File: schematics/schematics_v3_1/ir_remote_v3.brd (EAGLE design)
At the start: 77.5 x 49.5 mm, 26 parts, among them IC1 AP1117E50G, Q1 10MHz, T11 TASTER3301, T12 TASTER3301, T13 TASTER3301, T14 TASTER3301, T15 TASTER3301

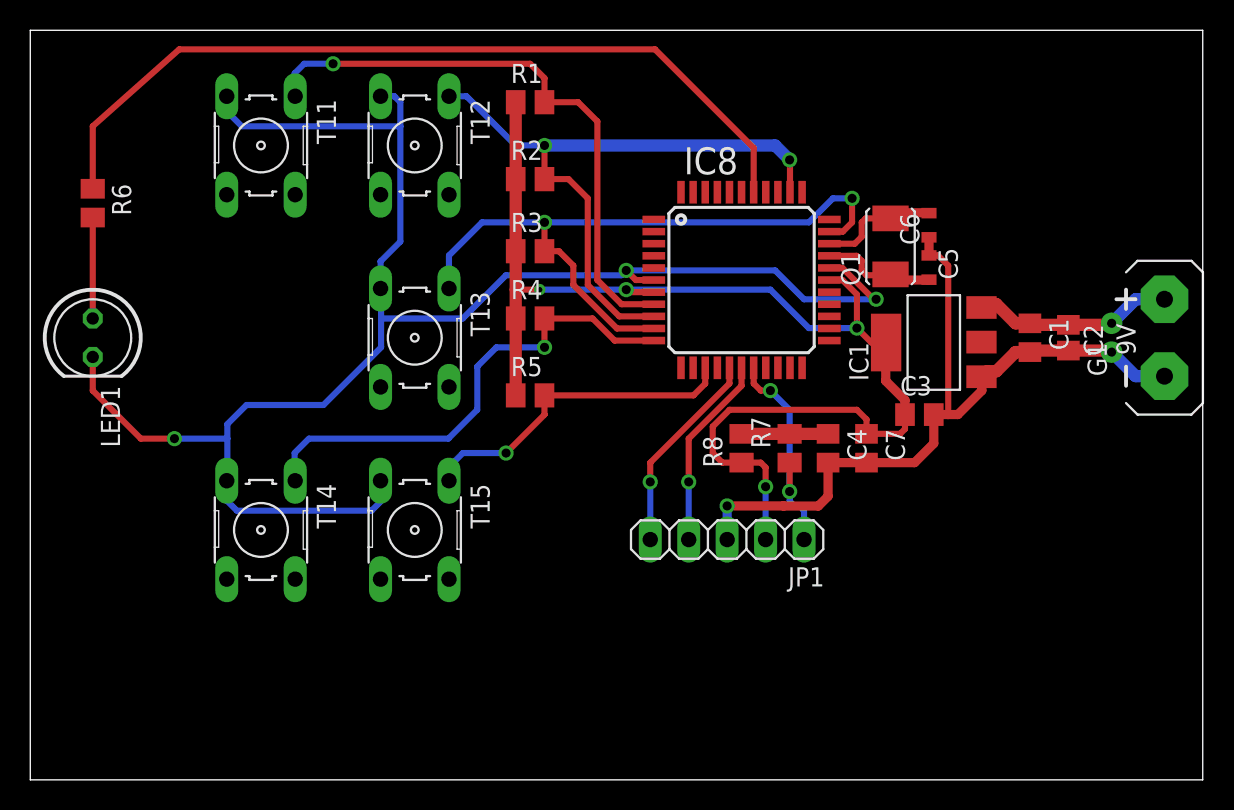
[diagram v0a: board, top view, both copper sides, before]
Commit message: Improve schematics v4
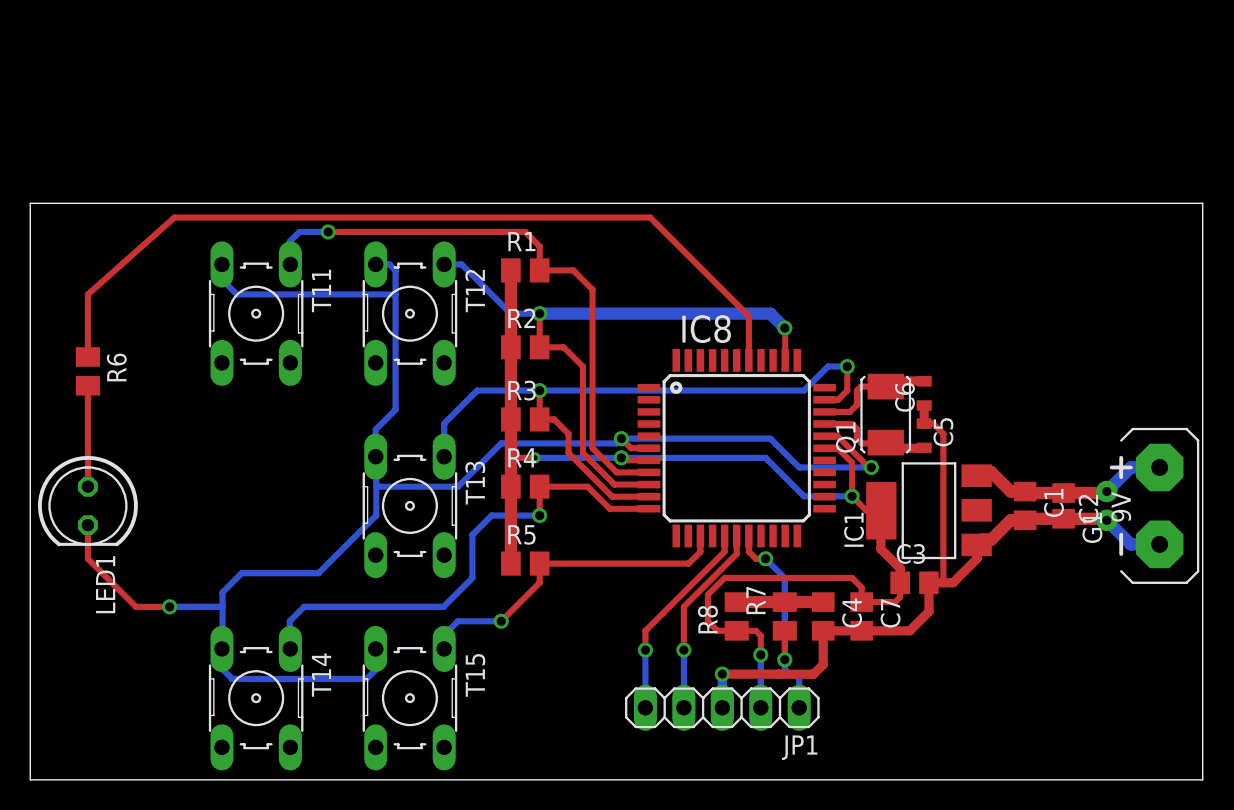
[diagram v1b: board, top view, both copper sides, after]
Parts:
- moved IC8 11.1 mm to (46.7, 21.9)
- moved C1 11.1 mm to (65.7, 18.1)
- moved C2 11.1 mm to (68.3, 18.1)
- moved C5 11.1 mm to (59.1, 22.7)
- moved G1 11.1 mm to (74.6, 18.1)
- moved JP1 11.1 mm to (45.7, 4.76)
- moved LED1 11.1 mm to (3.81, 18.1)
- moved Q1 11.1 mm to (56.5, 24.1)
- moved R2 11.1 mm to (32.7, 28.6)
- moved R4 11.1 mm to (32.7, 19.4)
- moved R6 11.1 mm to (3.81, 27.0)
- moved T13 11.1 mm to (25.1, 18.1)
- moved T14 11.1 mm to (14.9, 5.40)
- moved T15 11.1 mm to (25.1, 5.40)
- moved C3 11.1 mm to (58.4, 13.0)
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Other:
- board size 77.5 x 49.5 mm -> 77.5 x 38.1 mm
